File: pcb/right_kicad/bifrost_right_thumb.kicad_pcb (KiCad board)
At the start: 2 copper layers, 44.8 x 20.8 mm, 9 parts, among them J1 Conn_01x05, SW1 1U, SW2 1U

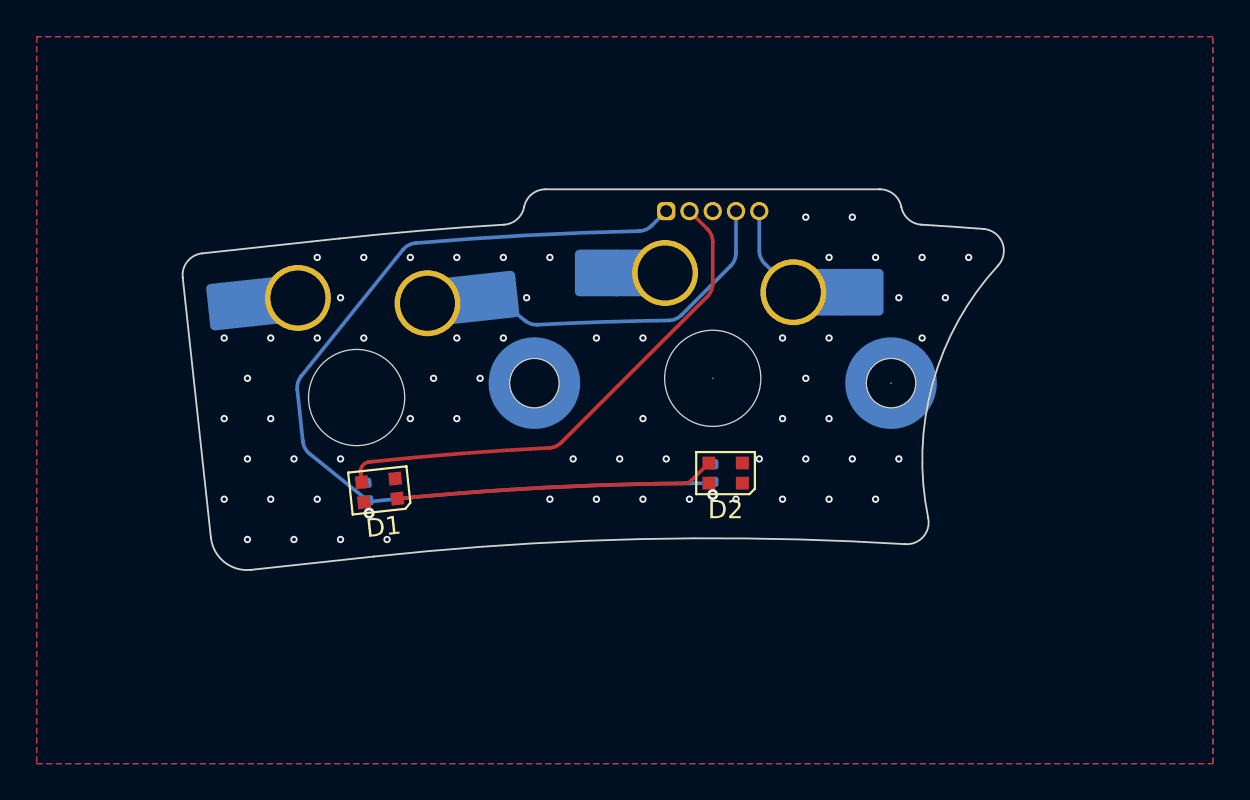
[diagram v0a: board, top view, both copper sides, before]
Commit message: Update PCB designs and fabrication outputs
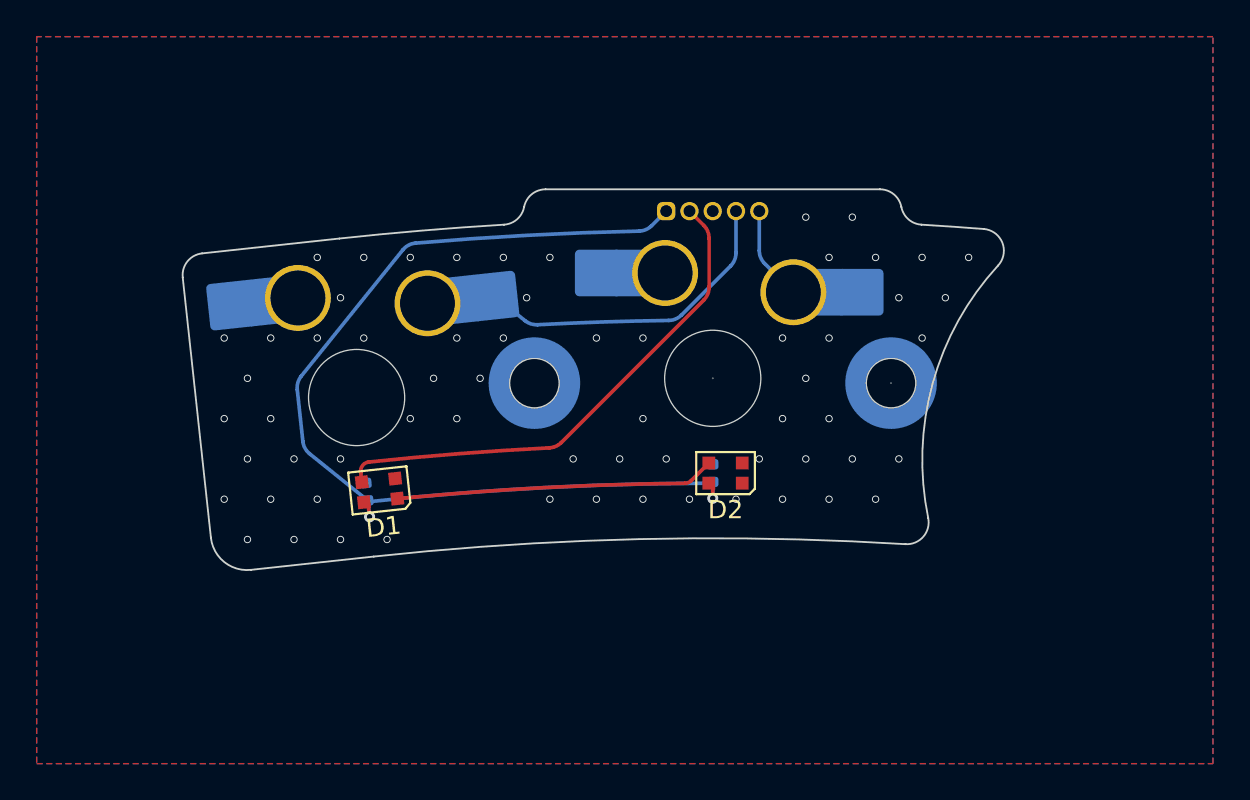
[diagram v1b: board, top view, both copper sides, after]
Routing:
- net RGB_PWR: track 53.9 -> 54.7 mm
